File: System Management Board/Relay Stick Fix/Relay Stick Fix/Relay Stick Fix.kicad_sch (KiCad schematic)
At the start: 9 parts, among them J1 Conn_02x04, Q1 NMOS

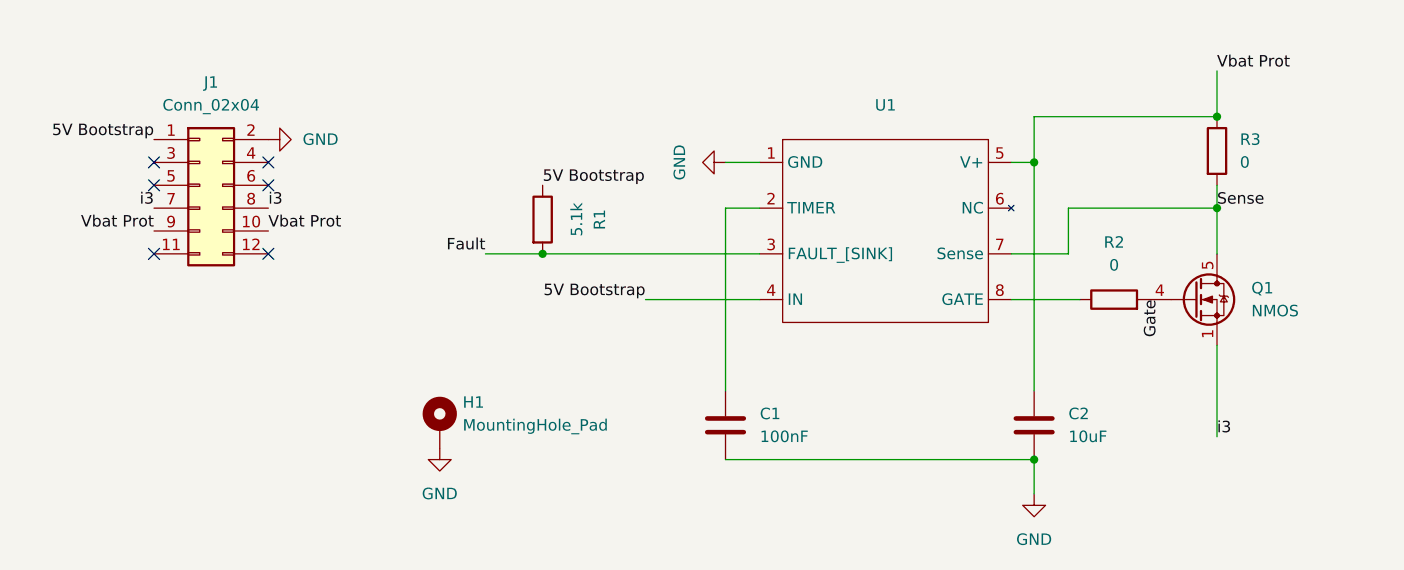
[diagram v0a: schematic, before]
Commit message: pwr routed, test points etc
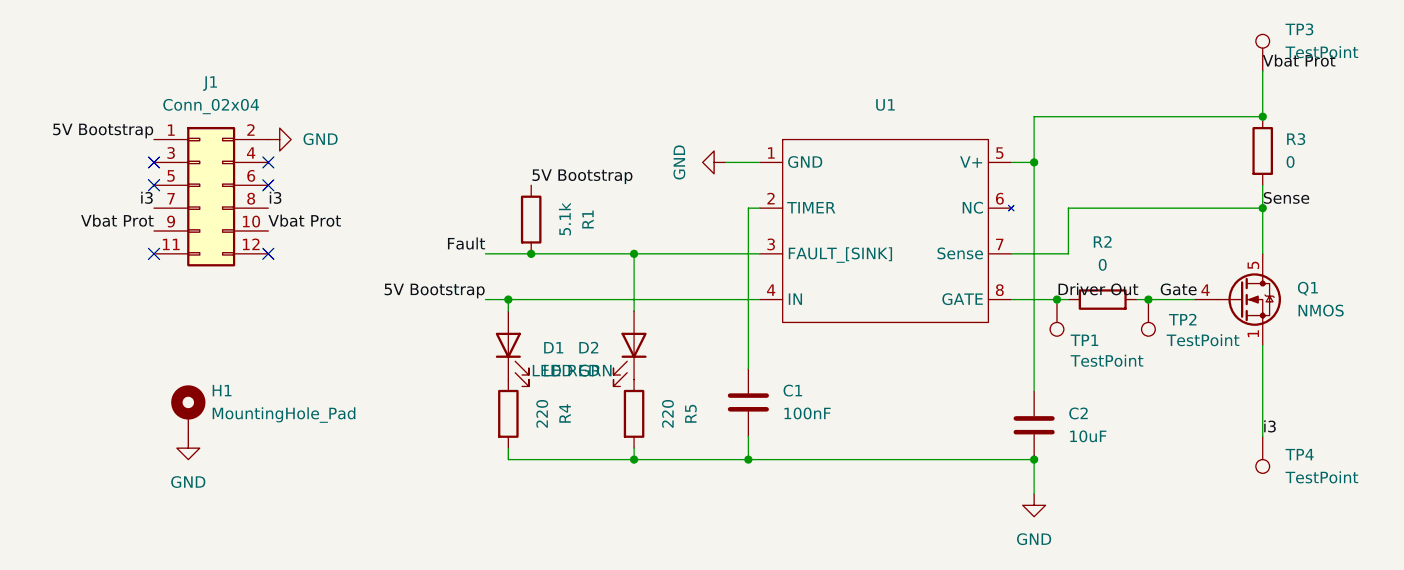
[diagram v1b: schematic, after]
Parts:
- added D1: LED GRN, LED_SMD:LED_1206_3216Metric_Pad1.42x1.75mm_HandSolder, symbol Device:LED
- added D2: LED RED, LED_SMD:LED_1206_3216Metric_Pad1.42x1.75mm_HandSolder, symbol Device:LED
- added R4, R5: 220, Resistor_SMD:R_1206_3216Metric_Pad1.30x1.75mm_HandSolder, symbol Device:R
- added TP1, TP2: TestPoint, TestPoint:TestPoint_Pad_D1.0mm, symbol Connector:TestPoint
- added TP3, TP4: TestPoint, TestPoint:TestPoint_THTPad_D1.0mm_Drill0.5mm, symbol Connector:TestPoint
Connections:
- net 5V Bootstrap: now also D1.2 (A)
- net Fault: now also D2.2 (A)
- net GND: now also R4.2, R5.2
- net Gate: now also Q1.4 (G), R2.2, TP2.1
- net Vbat Prot: now also TP3.1
- net i3: now also TP4.1
- net Driver Out: now reaches R2.1, U1.8 (GATE)
- net Driver Out: now also TP1.1
- new net: D2.1 (K), R5.1
- new net: D1.1 (K), R4.1
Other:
- moved on the sheet: C1, H1, Q1, R1, R2, R3
